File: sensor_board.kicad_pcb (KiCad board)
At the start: 2 copper layers, 77 x 53.5 mm, 9 parts, among them J1 Sensor0, J2 Sensor1

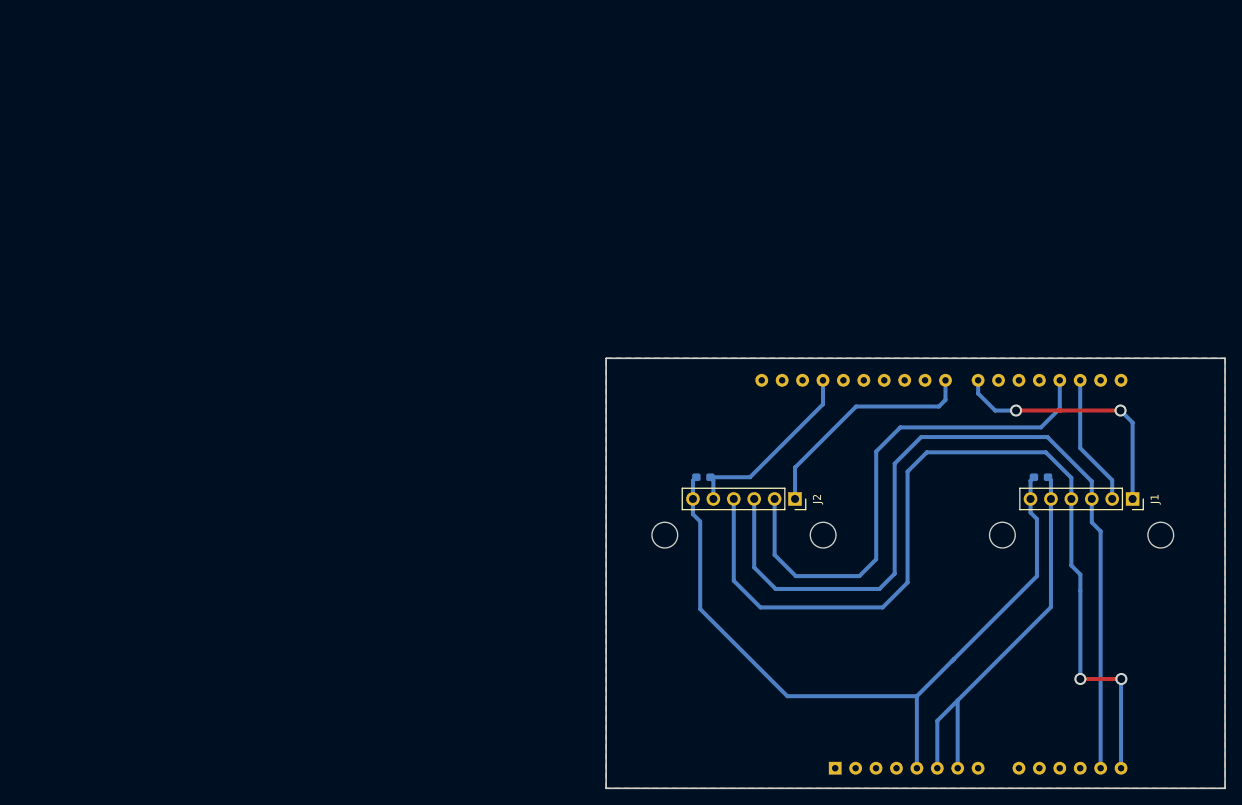
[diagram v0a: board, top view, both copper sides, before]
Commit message: made it teensy
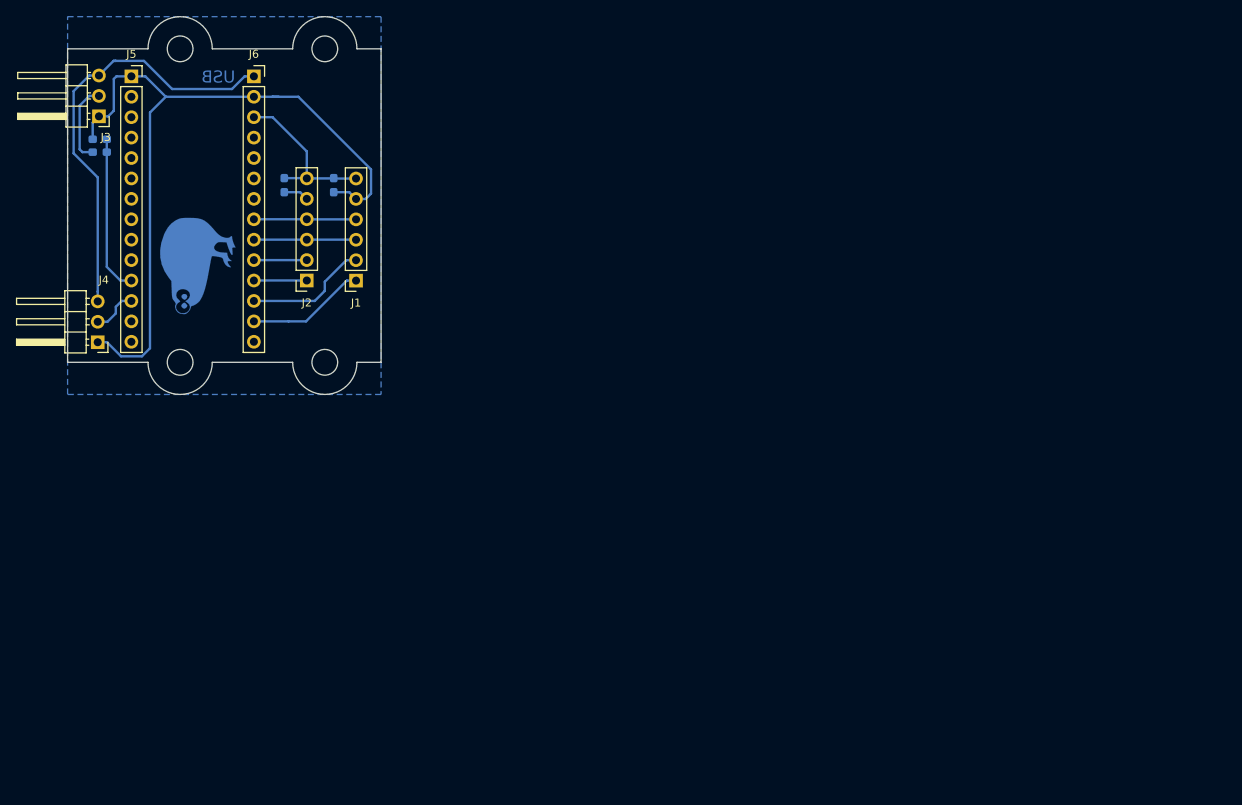
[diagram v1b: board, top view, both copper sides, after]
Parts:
- removed A1: Arduino_UNO_R3, Module:Arduino_UNO_R3
- removed the REF** at (180.0, 87.5)
- removed the REF** at (160.3, 87.5)
- removed the REF** at (138.0, 87.5)
- removed the REF** at (118.3, 87.5)
- added G***: LOGO, graphics:kiwi, F.Cu at (60.2, 54.0)
- added J3: iBUS-RX, Connector_PinHeader_2.54mm:PinHeader_1x03_P2.54mm_Horizontal, F.Cu at (47.9, 35.4)
- added J4: iBUS-TX, Connector_PinHeader_2.54mm:PinHeader_1x03_P2.54mm_Horizontal, F.Cu at (47.8, 63.5)
- added J5: teensyLeft, Connector_PinSocket_2.54mm:PinSocket_1x14_P2.54mm_Vertical, F.Cu at (51.9, 30.4)
- added J6: teensyRight, Connector_PinSocket_2.54mm:PinSocket_1x14_P2.54mm_Vertical, F.Cu at (67.2, 30.4)
- added R1: 11k5, Resistor_SMD:R_0603_1608Metric_Pad1.05x0.95mm_HandSolder, B.Cu at (48.0, 39.9)
- added R2: 22k1, Resistor_SMD:R_0603_1608Metric_Pad1.05x0.95mm_HandSolder, B.Cu at (48.0, 38.2)
- added REF**: MountingHole_3.2mm_M3, MountingHole:MountingHole_3.2mm_M3, F.Cu at (58.0, 66.0)
- added REF**: MountingHole_3.2mm_M3, MountingHole:MountingHole_3.2mm_M3, F.Cu at (58.0, 27.0)
- added REF**: MountingHole_3.2mm_M3, MountingHole:MountingHole_3.2mm_M3, F.Cu at (76.0, 27.0)
- added REF**: MountingHole_3.2mm_M3, MountingHole:MountingHole_3.2mm_M3, F.Cu at (76.0, 66.0)
- moved C2 100.9 mm to (71.0, 44.0), turned to 270 degrees
- moved J1 100.4 mm to (79.9, 55.8), turned to 180 degrees
- moved J2 66.5 mm to (73.8, 55.8), turned to 180 degrees
- moved C1 58.6 mm to (77.1, 44.0), turned to 270 degrees
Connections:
- net +5V renamed +3V3
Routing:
- net /SCL: track 112.7 -> 12.7 mm, vias 2 -> 0
- net /SDA: track 105.9 -> 12.7 mm
- net +3V3: track 91.7 -> 20.7 mm
- net /GPIO_1: track 63.5 -> 6.59 mm
- net +5V: track 0.00 -> 53.7 mm
- net GND: track 74.2 -> 98.1 mm
- net /~XSHUT_1: track 28.5 -> 6.59 mm
- net /iBUS-RX: track 0.00 -> 19.6 mm
- net /~XSHUT_0: track 32.2 -> 14.8 mm, vias 2 -> 0
- net Net-(J3-Pad2): track 0.00 -> 10.1 mm
- net /iBUS-TX: track 0.00 -> 5.74 mm
- net /GPIO_0: track 16.4 -> 15.5 mm
- removed copper zone on F.Cu, net GND
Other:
- board size 77 x 53.5 mm -> 39 x 47 mm
- board text added: "USB"
